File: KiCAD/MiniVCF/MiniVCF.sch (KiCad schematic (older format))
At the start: 45 parts, among them U1 TL074, U2 TL074

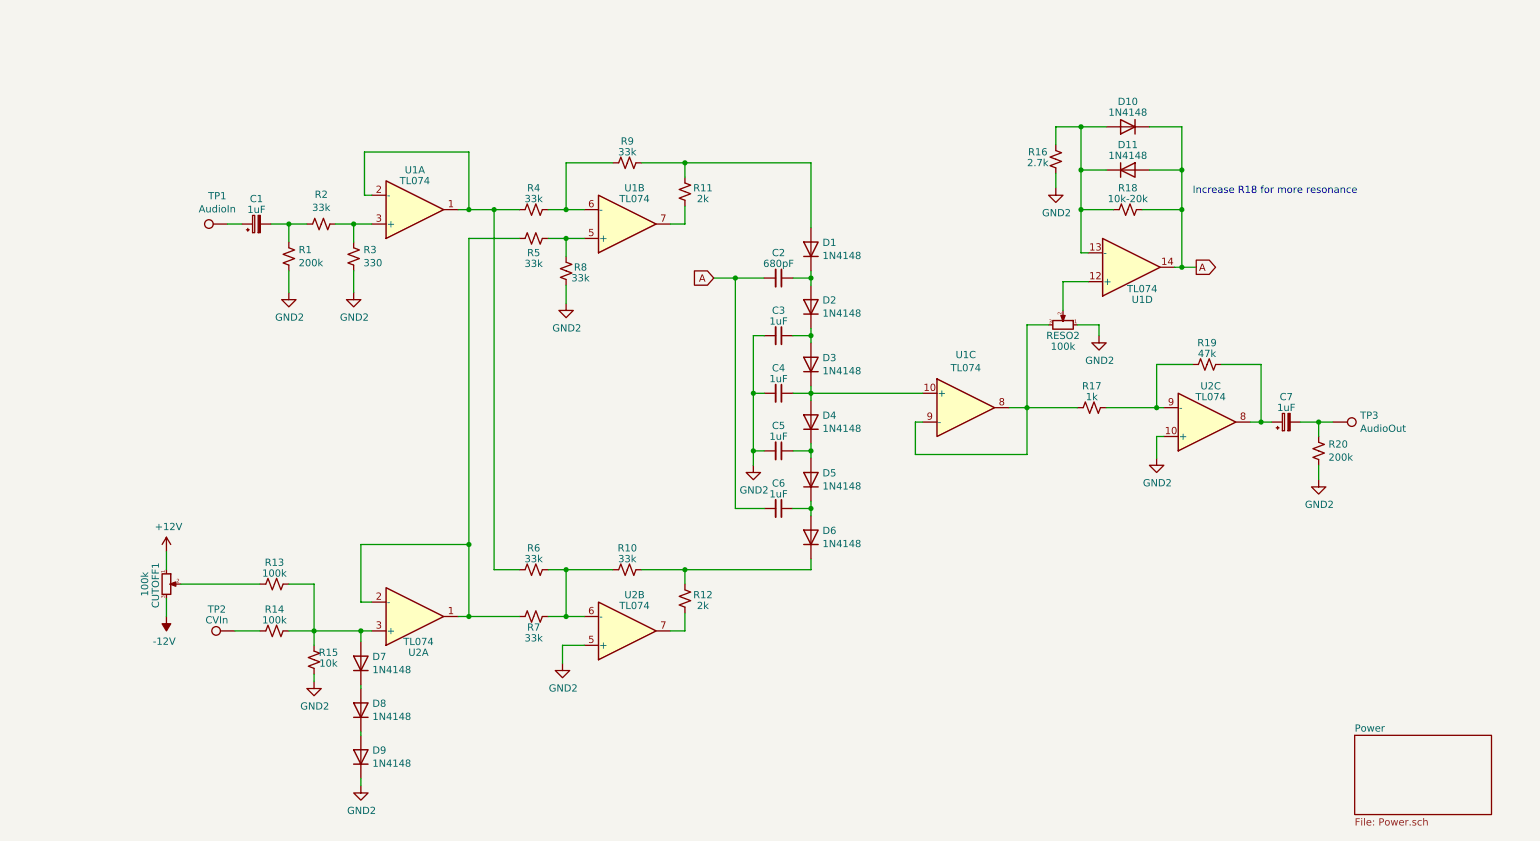
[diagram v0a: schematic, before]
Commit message: First pcb layout draft
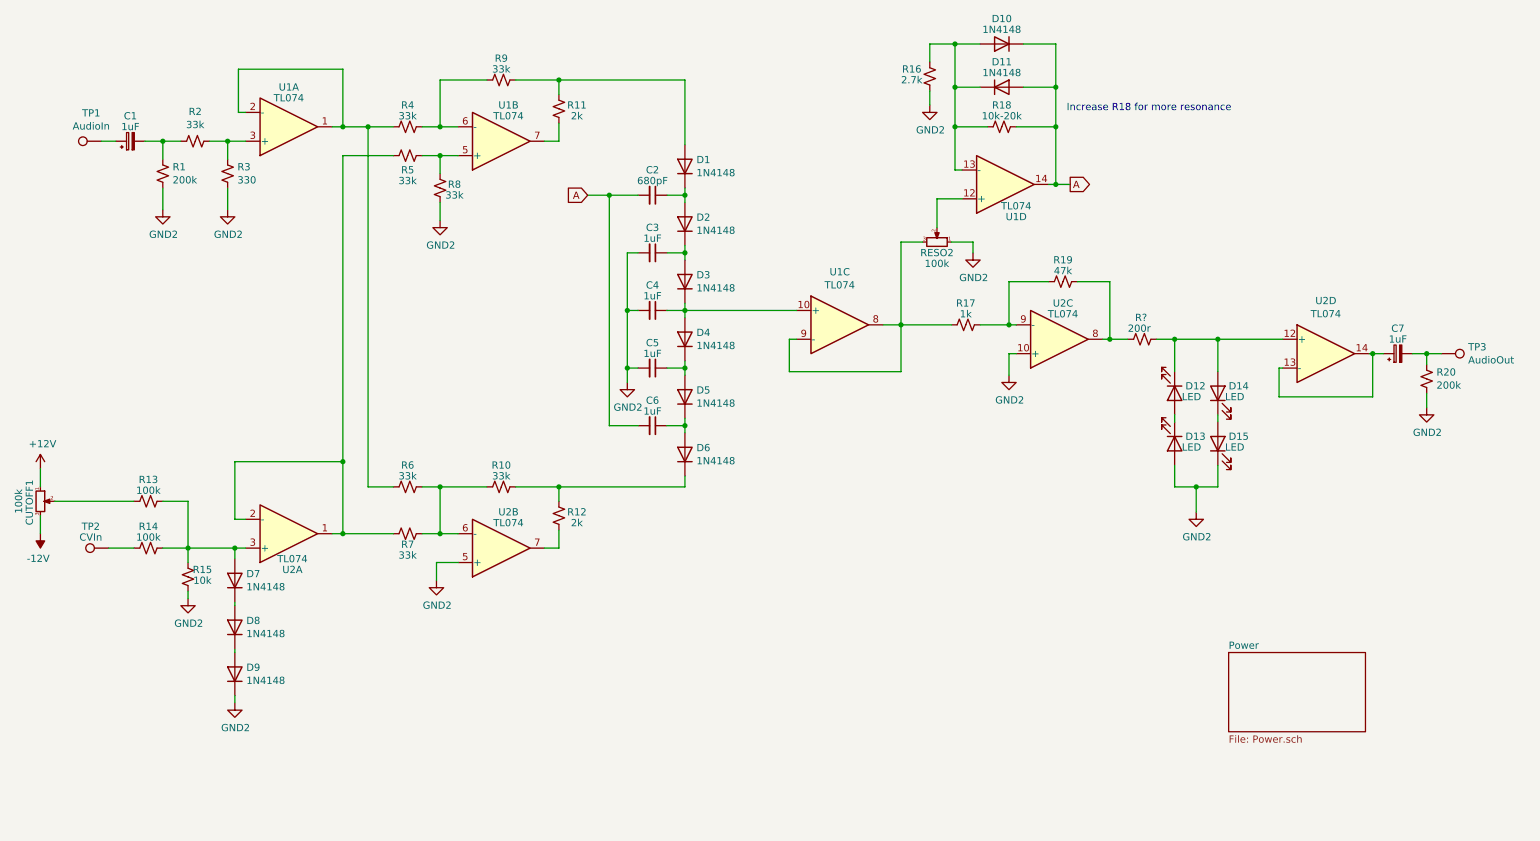
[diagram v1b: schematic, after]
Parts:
- added D12, D13, D14, D15: LED, symbol Device:LED
- added R?: 200r, symbol Device:R_Small_US
- added unit 4 of U2
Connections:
- net GND2: now also D13.2 (A), D15.1 (K)
- net at R19.2, U2.8: now also R?.2; no longer C7.1
- new net: D12.1 (K), D14.2 (A), R?.1, U2.12 (+)
- new net: D12.2 (A), D13.1 (K)
- new net: D14.1 (K), D15.2 (A)
- new net: C7.1, U2.13 (-), U2.14
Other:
- moved on the sheet: C1, C2, C3, C4, C5, C6, C7, CUTOFF1, D1, D10, D11, D2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
